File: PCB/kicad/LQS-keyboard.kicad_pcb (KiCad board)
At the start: 2 copper layers, 148.9 x 134.5 mm, 69 parts, among them SW1 SW_Push, SW10 SW_Push, SW11 SW_Push, SW12 SW_Push, SW13 SW_Push, SW14 SW_Push, SW15 SW_Push, SW16 SW_Push, SW17 SW_Push, SW18 SW_Push, SW19 SW_Push, SW2 SW_Push, SW20 SW_Push, SW21 SW_Push, SW22 SW_Push, SW23 SW_Push, SW24 SW_Push, SW25 SW_Push, SW26 SW_Push, SW27 SW_Push, SW28 SW_Push, SW29 SW_Push, SW3 SW_Push, SW4 SW_Push, SW5 SW_Push, SW6 SW_Push, SW7 SW_Push, SW8 SW_Push, SW9 SW_Push, U2 ProMicro

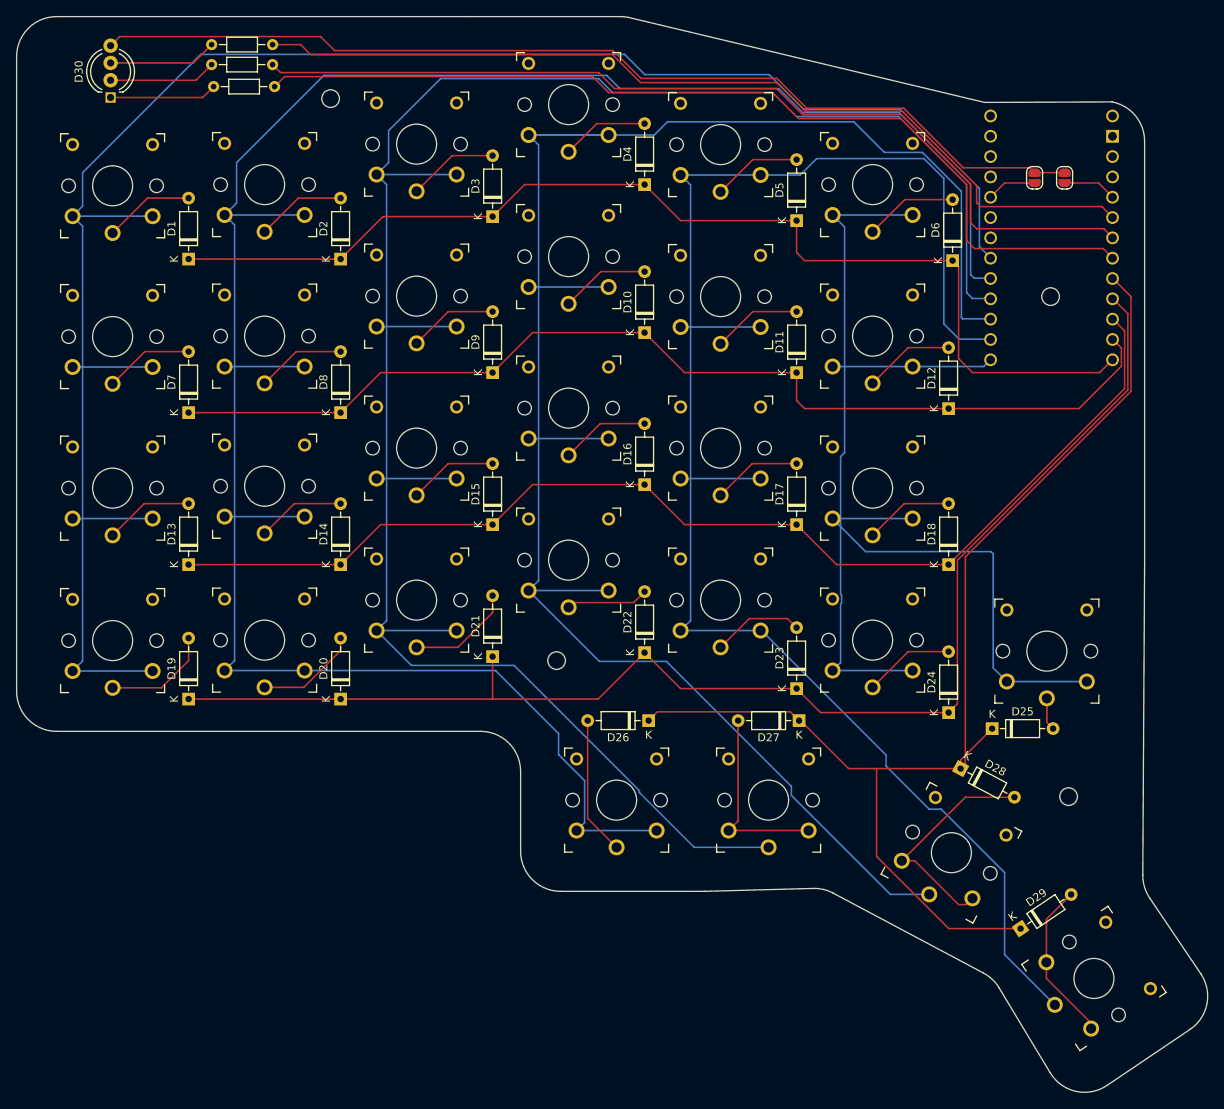
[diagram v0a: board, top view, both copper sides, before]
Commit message: 2025-07-07 update
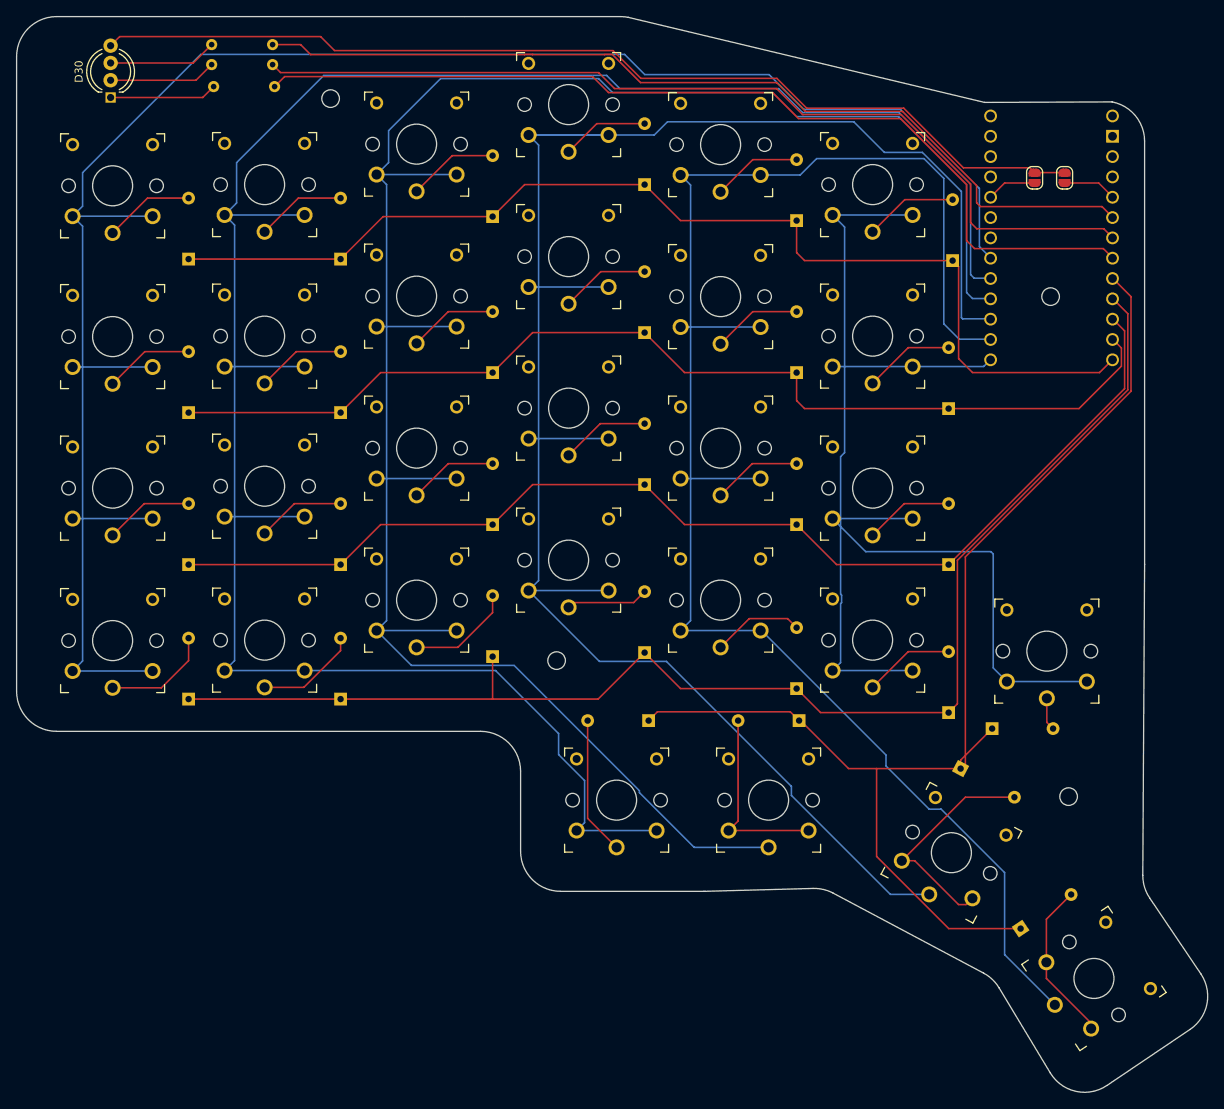
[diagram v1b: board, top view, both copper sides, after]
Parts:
- D1, D10, D11, D12, D13, D14, D15, D16, D17, D18, D19, D2, D20, D21, D22, D23, D24, D25, D26, D27, D28, D29, D3, D4, D5, D6, D7, D8, D9, R1, R2, R3: moved to B.Cu
